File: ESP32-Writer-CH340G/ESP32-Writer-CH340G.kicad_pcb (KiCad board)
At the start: 2 copper layers, 36.4 x 30.7 mm, 30 parts, among them J1 ESP-Prog-ProgramCOM-SEND, J2 USB2.0_C, J3 UART-OUTPUT, J4 USB2.0_C, Q1 2N7002, Q2 2N7002, U1 AMS1117-3.3, U2 CH340G, Y1 12M

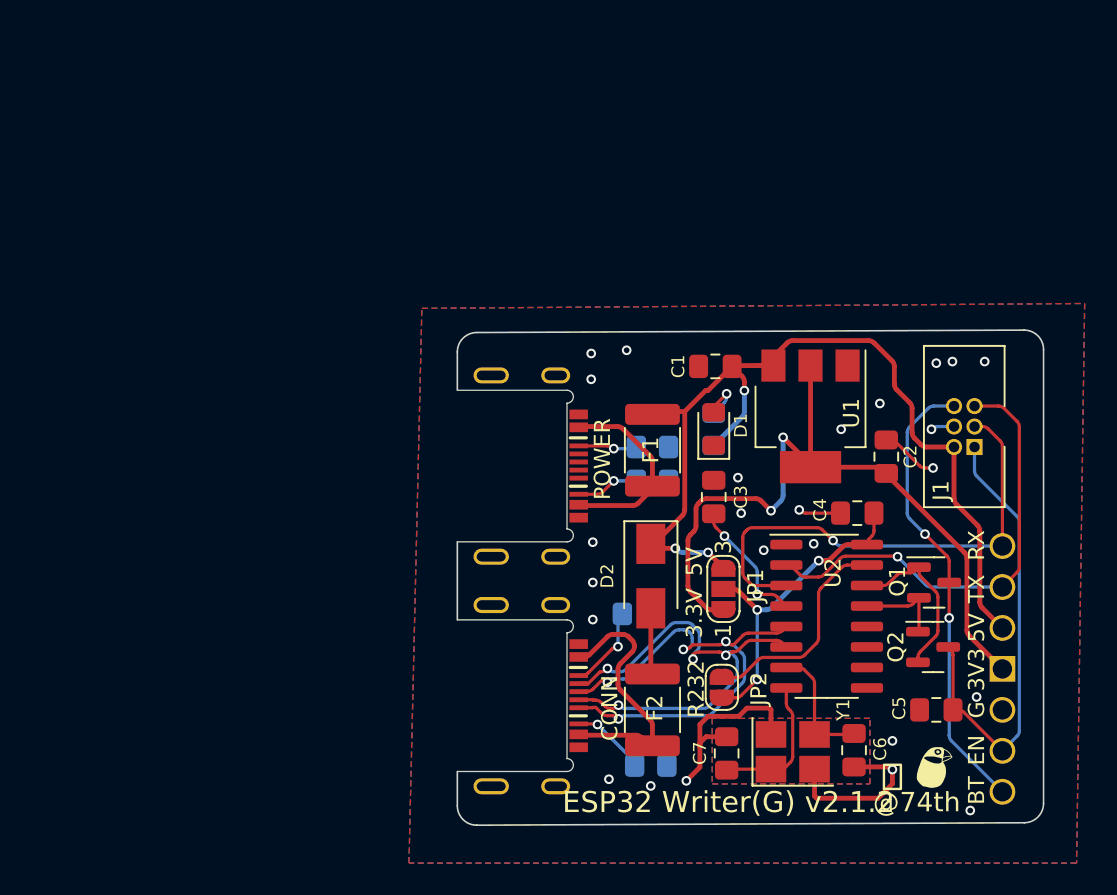
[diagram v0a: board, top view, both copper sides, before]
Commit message: esp32-writer/v3.0.0
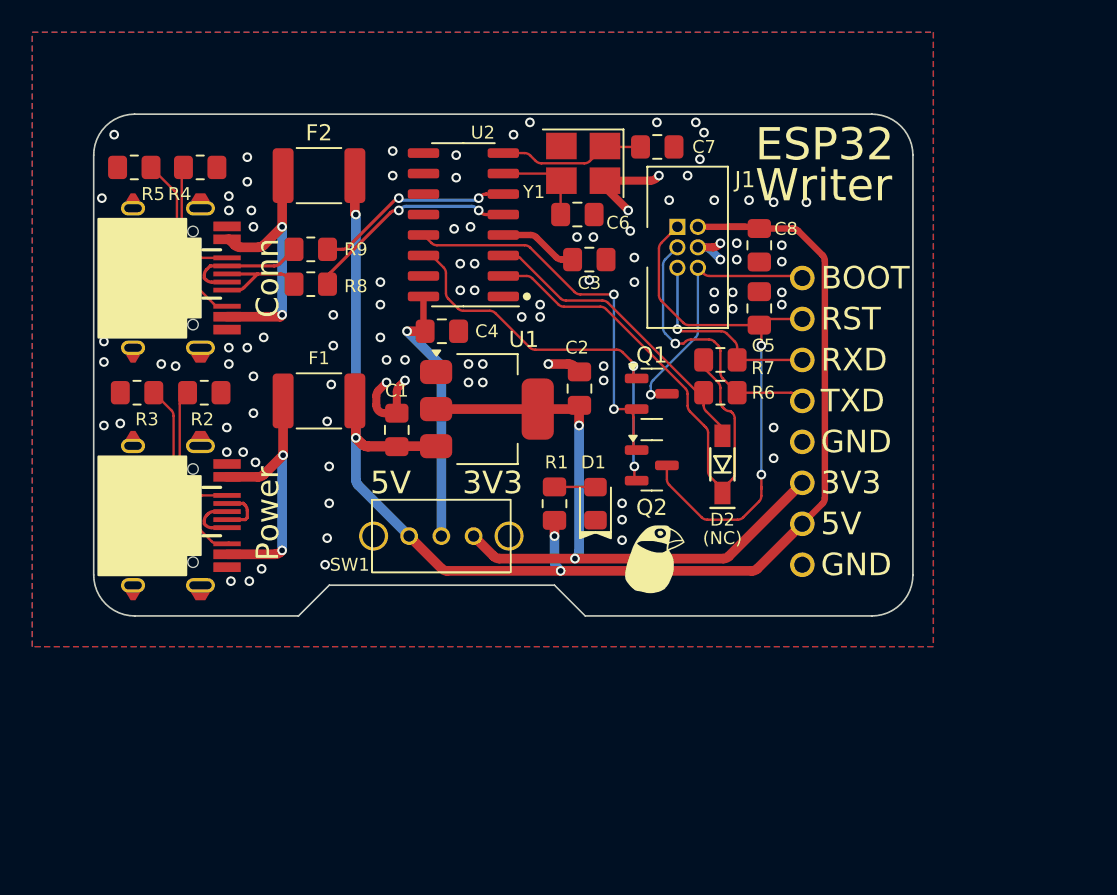
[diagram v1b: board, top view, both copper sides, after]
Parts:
- removed G***: LOGO, $74th:74th-3mm
- removed JP1: Jumper_3_Open, Jumper:SolderJumper-3_P1.3mm_Open_RoundedPad1.0x1.5mm_NumberLabels
- removed JP2: Jumper_2_Open, Jumper:SolderJumper-2_P1.3mm_Open_RoundedPad1.0x1.5mm
- removed the REF** at (95.2, 96.0)
- added C8: 22u, 74th:Capacitor_0805_2012, F.Cu at (85.7, 56.4)
- added MISC-ICON: LOGO, 74th:Logo_74th_5mm, F.Cu at (79.1, 76.1)
- added R6: 10(470), 74th:Capacitor_0805_2012, F.Cu at (83.3, 65.5)
- added R7: 10, 74th:Capacitor_0805_2012, F.Cu at (83.3, 63.5)
- added R8: 10, 74th:Register_0805_2012, F.Cu at (57.9, 58.8)
- added R9: 10, 74th:Register_0805_2012, F.Cu at (57.9, 56.6)
- added REF**: JLCJLCJLCJLC, 74th:Logo_JLCJLCJLCJLC, B.Cu at (88.1, 78.4)
- added SW1: SK-12D02-G020, 74th:Switch_Slide_SK-12D02-G020, F.Cu at (66.0, 74.4)
- C1, C2, C3, C5, C6, C7: footprint $74th:Capacitor_0805_2012 -> 74th:Capacitor_0805_2012
- C4: value 100nF -> 100n; footprint $74th:Capacitor_0805_2012 -> 74th:Capacitor_0805_2012
- D1: value LED -> BLUE; footprint $74th:LED_0805_2012Metric_Pad1.15x1.40mm_HandSolder -> 74th:LED_0805_2012
- D2: value D_Schottky -> NC(1N4148W); footprint $74th:D_SMA -> 74th:Package_SOD23_Diode
- F1, F2: footprint $74th:Fuse_1812_4532Metric_Pad1.30x3.40mm_HandSolder -> 74th:Package_Fuse_1812_4532m
- J2, J4: footprint $74th:USB-C-12-Pin-MidMount-ali-v5 -> 74th:Connector_USB-C-Receptacle_SMT_12-Pin_Simple
- J3: footprint esp32-dev-board:UART -> 74th:PinOut_Pin_8
- R1: value 200 -> 10k; footprint $74th:Register_0805_2012 -> 74th:Register_0805_2012; moved to F.Cu
- R2, R3, R4, R5: footprint $74th:Register_0805_2012 -> 74th:Register_0805_2012; moved to F.Cu
- U2: footprint Package_SO:SOP-16_3.9x9.9mm_P1.27mm -> 74th:Package_SOIC-16_3.9x9.9mm_P1.27mm
- Y1: footprint $74th:Crystal_SMD_3225-4Pin_3.2x2.5mm_HandSoldering -> 74th:Crystal_SMD_3225-4Pin_3.2x2.5mm_HandSoldering
- moved R5 49.0 mm to (47.0, 51.6), turned to 180 degrees
- moved F2 39.1 mm to (58.4, 52.1), turned to 0 degrees
- moved R4 38.8 mm to (51.1, 51.6)
- moved Y1 38.7 mm to (74.8, 51.3), turned to 180 degrees
- moved C7 37.9 mm to (79.4, 50.3), turned to 180 degrees
- moved C6 37.4 mm to (74.4, 54.5), turned to 180 degrees
- moved U2 33.1 mm to (67.4, 55.1), turned to 180 degrees
- moved J4 32.7 mm to (47.0, 58.4)
- moved R3 32.4 mm to (47.1, 65.5), turned to 180 degrees
- moved C4 28.1 mm to (66.0, 61.7), turned to 0 degrees
- moved R2 28.0 mm to (51.3, 65.5)
- moved C5 27.2 mm to (85.7, 60.3), turned to 90 degrees
- moved Q1 21.1 mm to (79.1, 65.6)
- moved F1 20.9 mm to (58.4, 66.0), turned to 0 degrees
- moved Q2 20.8 mm to (79.1, 70.0)
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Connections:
- net DTR renamed /DTR
- net Net-(JP1-C) renamed VCC
- net RTS renamed /RTS
- C5 pad 1: RESET -> /RESET
- D2 pad 1: +5V -> Net-(D2-K)
- F2 pad 2: Net-(D2-A) -> +5V
- J1 pad 1: RESET -> /RESET
- J1 pad 3: RXD -> /RXD
- J1 pad 5: TXD -> /TXD
- J1 pad 6: BOOT -> /BOOT
- J3 pad 1: RXD -> GND
- J3 pad 2: TXD -> +5V
- J3 pad 3: +5V -> +3V3
- J3 pad 4: +3V3 -> GND
- J3 pad 5: GND -> /RXD
- J3 pad 6: RESET -> /TXD
- J3 pad 7: BOOT -> /RESET
- J4 pad 2: UD- -> Net-(J4-D-)
- J4 pad 3: UD+ -> Net-(J4-D+)
- Q1 pad 3: BOOT -> /BOOT
- Q2 pad 3: RESET -> /RESET
- U2 pad 15: Net-(JP2-B) -> unconnected-(U2-R232-Pad15)
- U2 pad 2: TXD -> Net-(D2-K)
- U2 pad 3: RXD -> Net-(D2-A)
- U2 pad 5: UD+ -> /DP
- U2 pad 6: UD- -> /DM
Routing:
- net /RESET: track 0.00 -> 34.0 mm, vias 0 -> 2
- net UD+: track 31.6 -> 0.00 mm, vias 4 -> 0
- net +5V: track 58.9 -> 90.4 mm, vias 3 -> 4
- net UD-: track 30.7 -> 0.00 mm, vias 4 -> 0
- net RXD: track 30.6 -> 0.00 mm, vias 1 -> 0
- net Net-(D2-K): track 0.00 -> 30.1 mm
- net TXD: track 28.6 -> 0.00 mm, vias 1 -> 0
- net RESET: track 28.4 -> 0.00 mm
- net BOOT: track 28.3 -> 0.00 mm, vias 2 -> 0
- net /DTR: track 5.54 -> 23.9 mm, vias 0 -> 2
- net /BOOT: track 0.00 -> 17.4 mm, vias 0 -> 1
- net /RXD: track 0.00 -> 17.1 mm, vias 0 -> 1
- net Net-(D2-A): track 3.94 -> 19.2 mm
- net /RTS: track 10.4 -> 24.7 mm, vias 0 -> 2
- net Net-(JP2-B): track 14.2 -> 0.00 mm
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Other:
- board size 36.4 x 30.7 mm -> 50.8 x 31.1 mm
- board text added: "(NC)"
- board text added: "3V3"
- board text added: "5V"
- board text added: "74TH-G045-3.0.0"
- board text added: "BOOT"
- board text added: "Conn"
- board text added: "ESP32"
- board text added: "GND"
- board text added: "Power"
- board text added: "RST"
- board text added: "RXD"
- board text added: "TXD"
- board text added: "Writer"
- board text removed: "CONN"
- board text removed: "ESP32 Writer(G) v2.1.2"
- board text removed: "JLCJLCJLCJLC"
- board text removed: "POWER"
- board text removed: "R232"
